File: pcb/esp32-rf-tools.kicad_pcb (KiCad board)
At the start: 2 copper layers, 120 x 75 mm, 7 parts, among them U1 ESP32-WROOM-32UE, U2 NRF24L01_Breakout, U3 TP4056_Module_Protected, U4 CC1101, U5 NRF24L01_Breakout

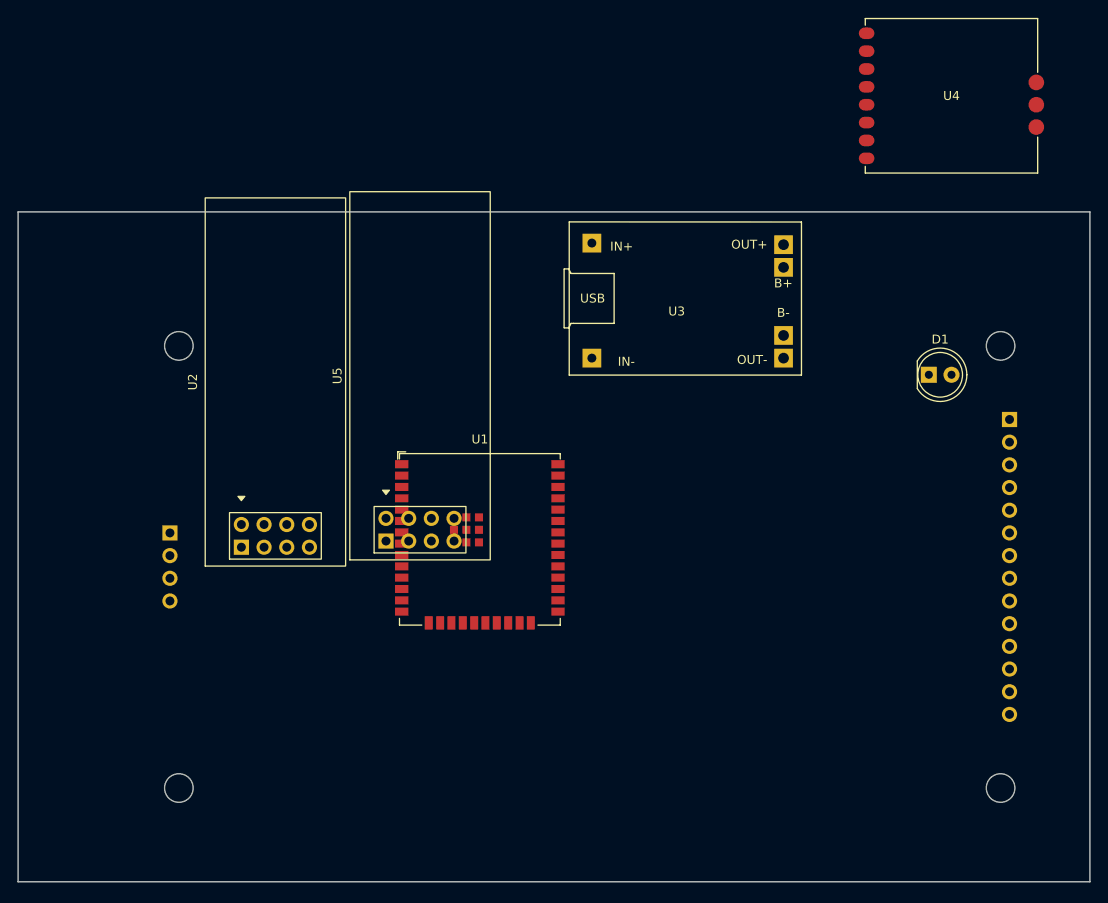
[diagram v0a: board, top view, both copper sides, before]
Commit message: m2
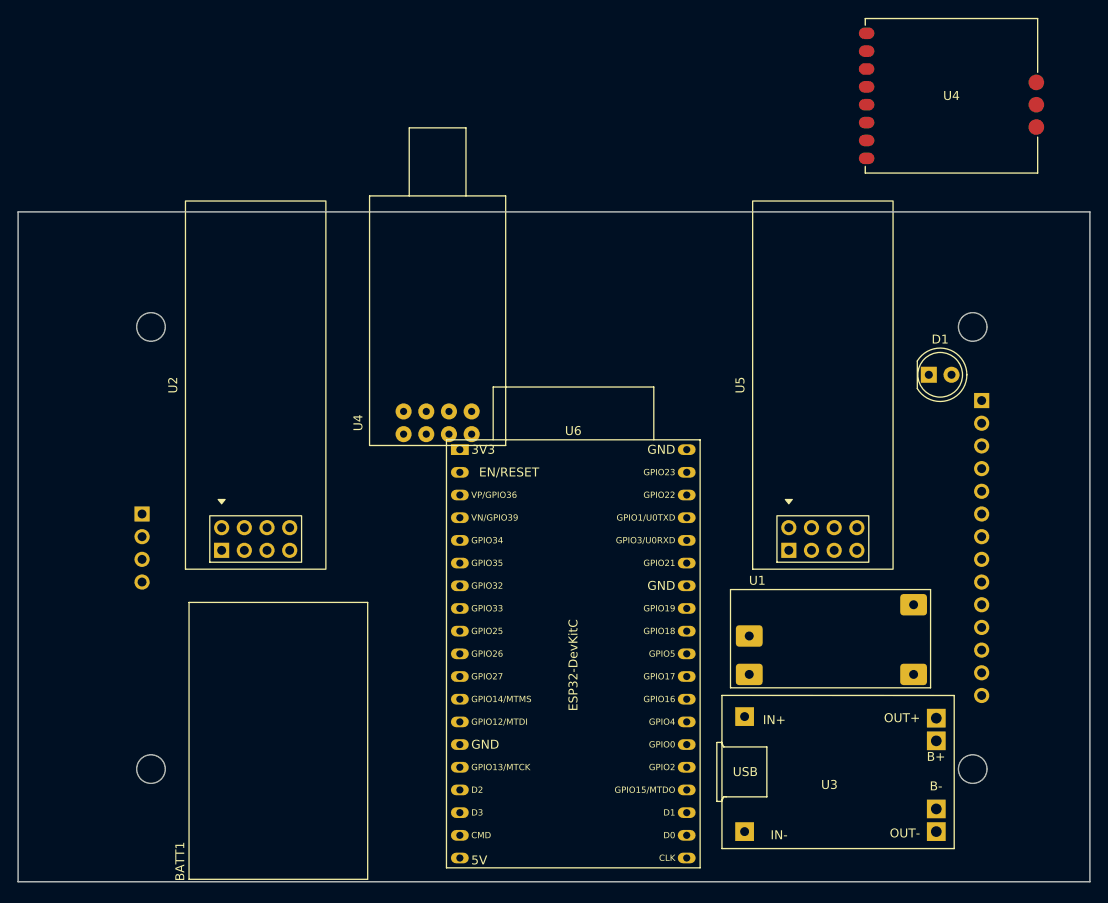
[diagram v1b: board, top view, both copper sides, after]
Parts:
- added BATT1: Battery 3.7v 550mAh, truke:Battery 902030, F.Cu at (101.1, 114.7)
- added U4: ~, truke:CC1101 433 MHz, F.Cu at (129.6, 50.8)
- added U6: ESP32-DevKitC, PCM_Espressif:ESP32-DevKitC, F.Cu at (124.5, 76.6)
- U1: value ESP32-WROOM-32UE -> Step-up 3.7 - 12V; footprint esp32-rf-tools:ESP32-WROOM-32UE -> truke:Step-up_3.7_12
- moved U3 55.7 mm to (167.1, 113.0)
- moved U5 45.1 mm to (161.3, 87.9)
- moved U1 38.5 mm to (161.8, 102.5)
- moved DS1 3.77 mm to (182.9, 71.1)
- moved U2 2.24 mm to (97.8, 87.9)
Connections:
- U1 pad 1: Net-(U1-GND-Pad1) -> unconnected-(U1-IN+-Pad1)
